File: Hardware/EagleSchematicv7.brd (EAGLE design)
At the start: 20.3 x 49.2 mm, 6 parts

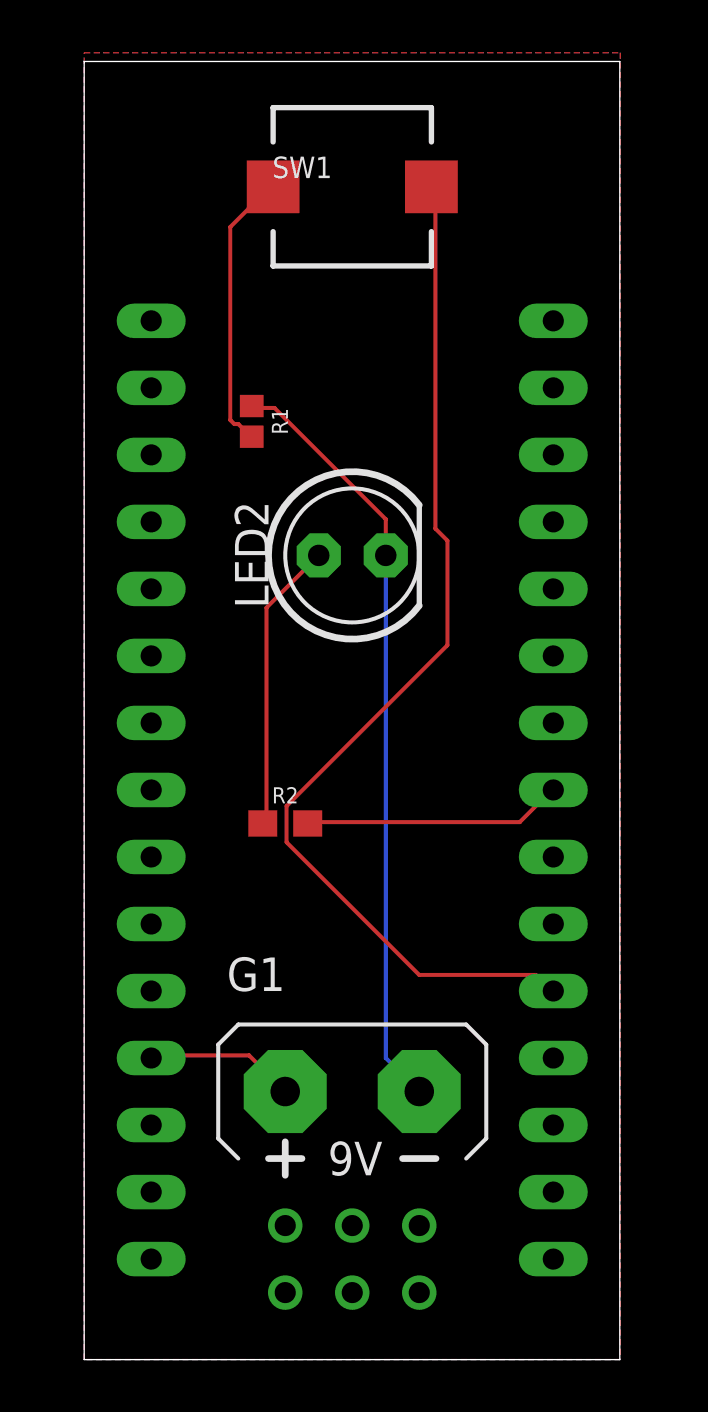
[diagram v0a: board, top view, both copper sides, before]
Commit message: Add files via upload
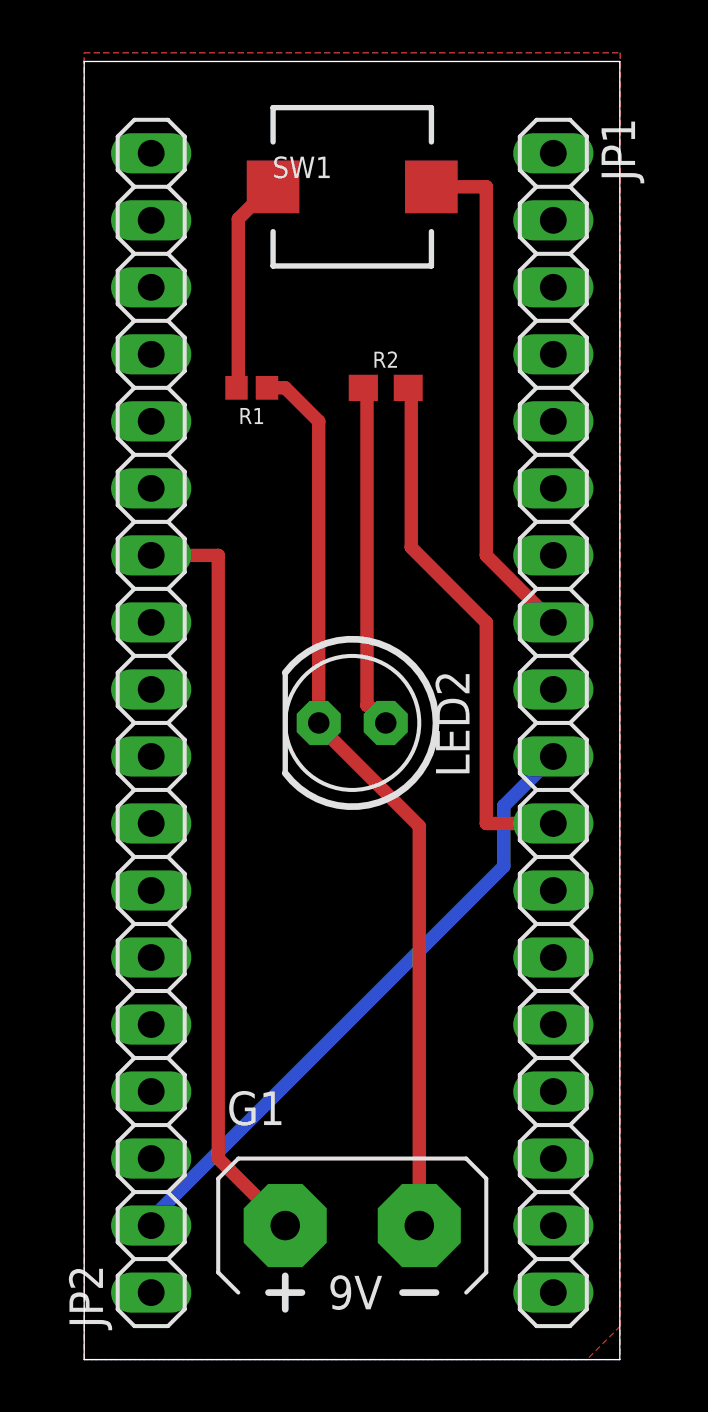
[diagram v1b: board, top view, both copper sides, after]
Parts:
- removed U$1: NANO, Arduino-clone:NANO
- added JP1, JP2: (no value), adafruit:1X18
- moved R2 16.9 mm to (14.0, 38.1)
- moved LED2 6.35 mm to (12.7, 25.4), turned to 180 degrees
- moved G1 5.08 mm to (12.7, 6.35)
- moved R1 1.27 mm to (8.89, 38.1), turned to 180 degrees
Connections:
- new net N$6: JP1.10, JP2.2
- net N$1: now also JP2.12; no longer U$1.5V
- net N$3: now also JP1.8; no longer U$1.D2
- net N$4: now also JP1.11; no longer U$1.D5
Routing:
- net N$6: track 0.00 -> 24.1 mm
- net N$1: track 5.69 -> 29.1 mm
- net N$3: track 40.2 -> 19.6 mm
- net N$4: track 9.83 -> 20.5 mm
- net GND: track 29.1 -> 34.5 mm
- net N$2: track 10.6 -> 8.30 mm
- net N$5: track 11.1 -> 13.3 mm
